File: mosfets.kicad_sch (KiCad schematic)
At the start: 25 parts, among them IC2 IRFR9014PBF, J4 Screw_Terminal_01x02, J5 Screw_Terminal_01x02, J6 Screw_Terminal_01x02, J7 Screw_Terminal_01x02, J8 Screw_Terminal_01x02, J9 Screw_Terminal_01x02, Q1 IRLML6244, Q2 IRLML6244, Q3 IRLML6244, Q4 IRLML6244, Q5 IRLML6244, Q6 IRLML6244

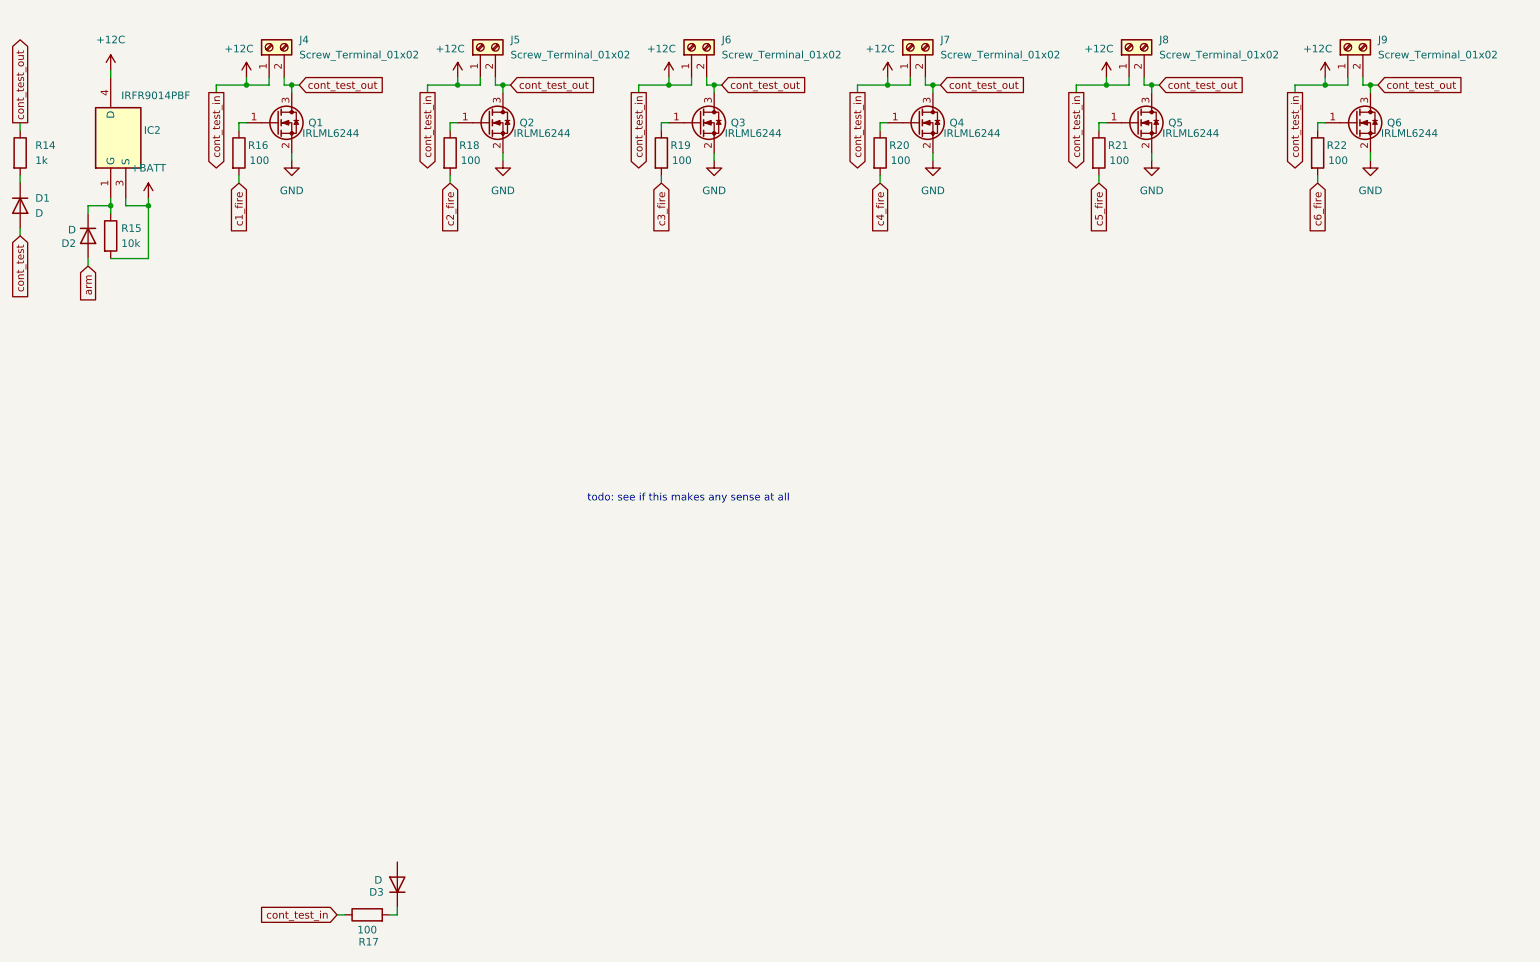
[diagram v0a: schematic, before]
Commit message: worked mainly on pcb
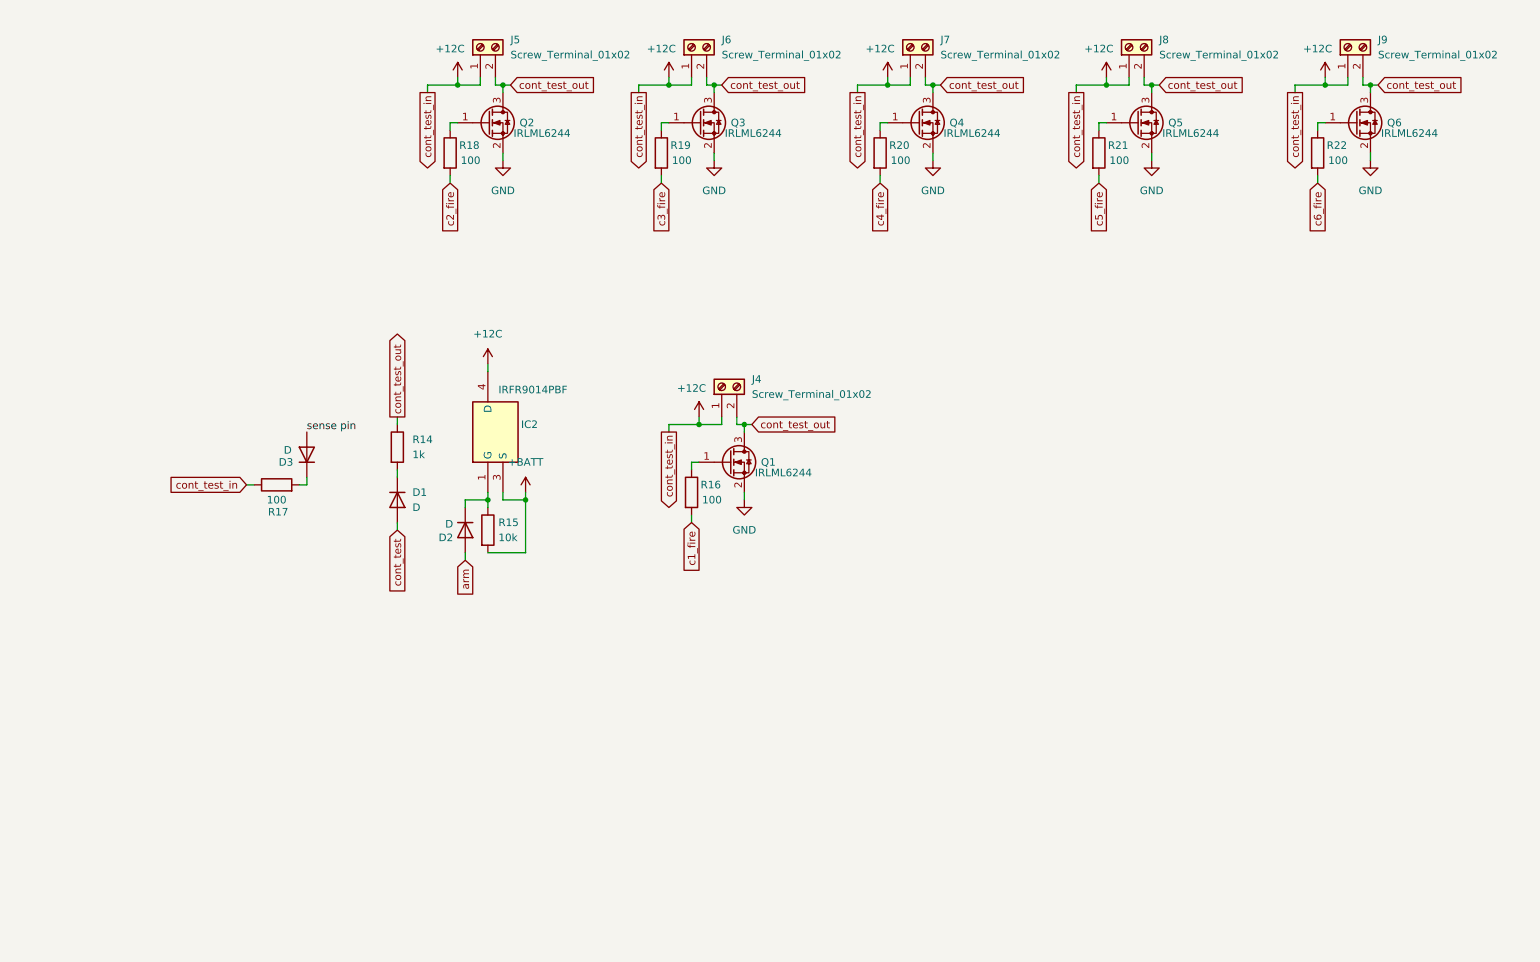
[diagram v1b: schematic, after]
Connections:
- net sense pin: now reaches D3.2 (A)
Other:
- note removed: "todo: see if this makes any sense at all"
- moved on the sheet: D1, D2, D3, IC2, J4, Q1, R14, R15, R16, R17
